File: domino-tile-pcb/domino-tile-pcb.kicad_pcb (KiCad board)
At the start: 2 copper layers, 39 x 35 mm, 1 part

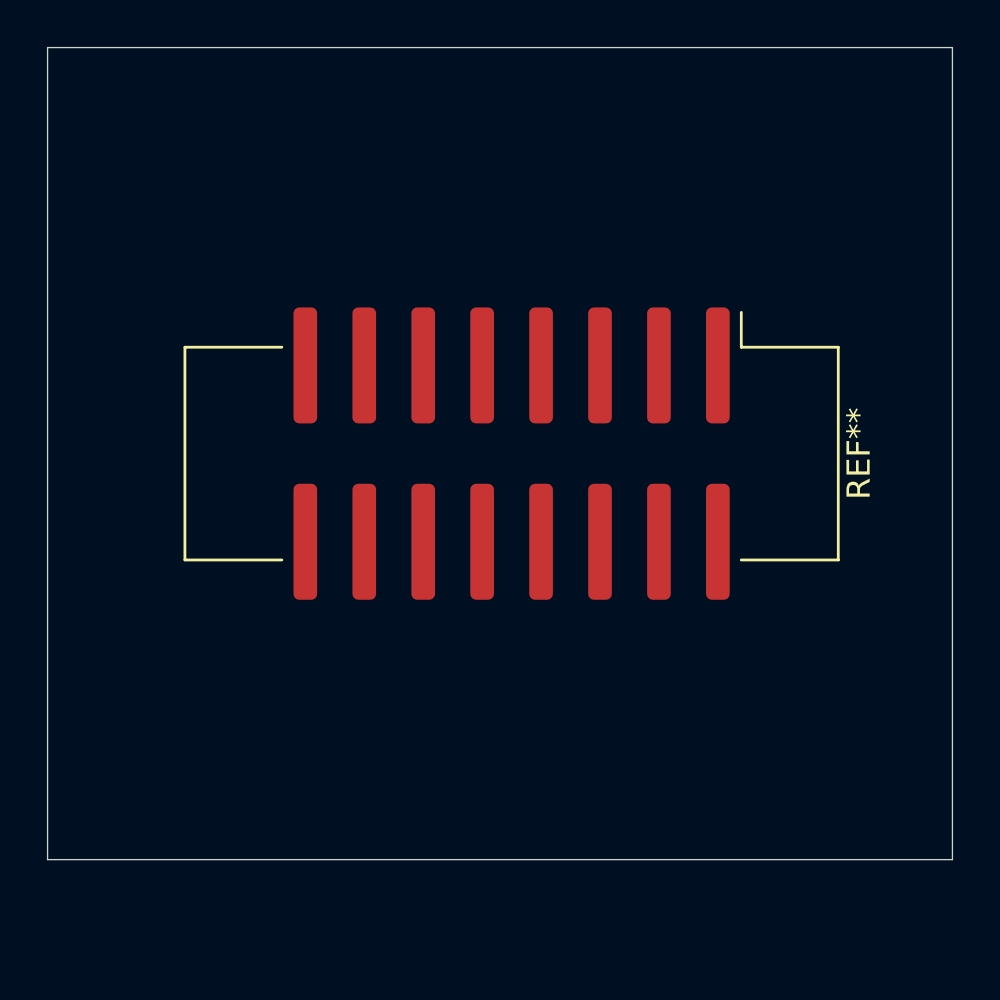
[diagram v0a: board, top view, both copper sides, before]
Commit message: do a lot of things, I guess
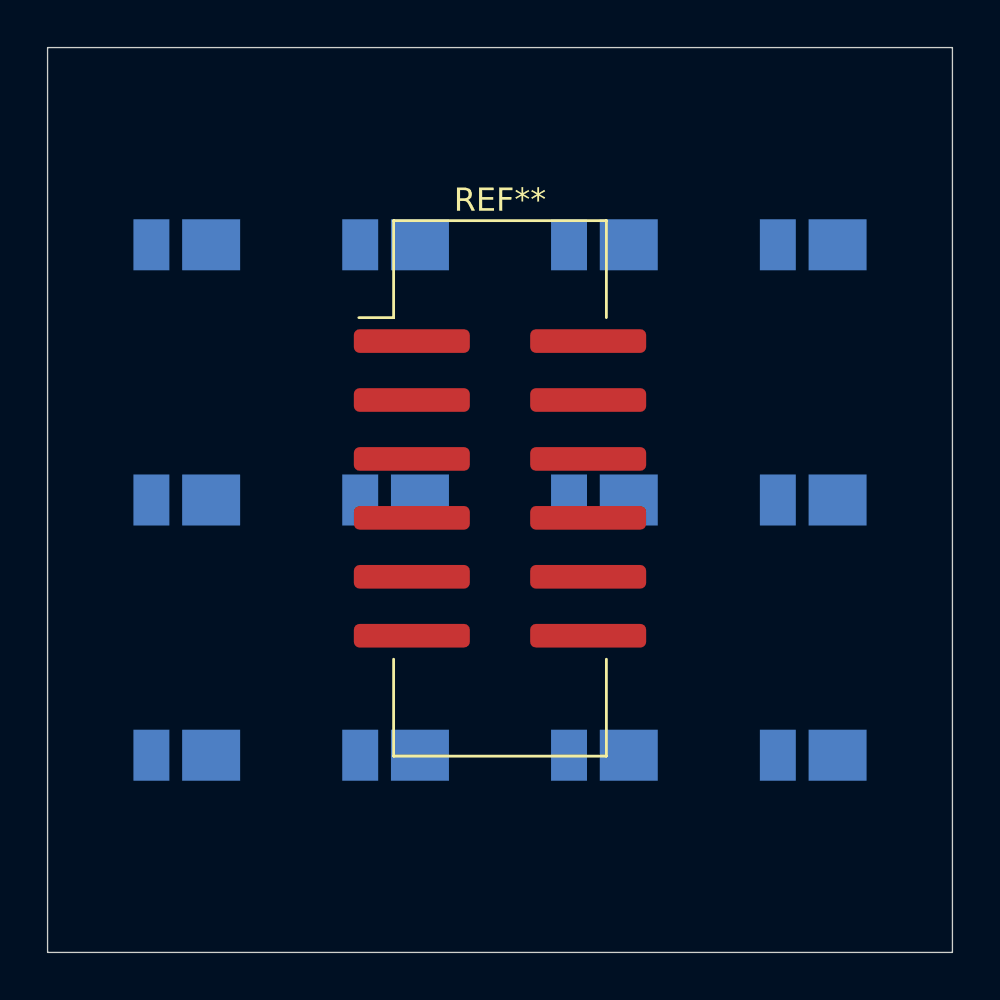
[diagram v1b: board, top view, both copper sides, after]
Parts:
- removed the REF** at (70.0, 67.5)
- added ?: 1, LED_SMD:LED_PLCC_2835_Handsoldering, B.Cu at (56.0, 69.5)
- added ?: 1, LED_SMD:LED_PLCC_2835_Handsoldering, B.Cu at (83.0, 58.5)
- added ?: 1, LED_SMD:LED_PLCC_2835_Handsoldering, B.Cu at (56.0, 58.5)
- added ?: 1, LED_SMD:LED_PLCC_2835_Handsoldering, B.Cu at (74.0, 58.5)
- added ?: 1, LED_SMD:LED_PLCC_2835_Handsoldering, B.Cu at (56.0, 80.5)
- added ?: 1, LED_SMD:LED_PLCC_2835_Handsoldering, B.Cu at (65.0, 58.5)
- added ?: 1, LED_SMD:LED_PLCC_2835_Handsoldering, B.Cu at (74.0, 80.5)
- added ?: 1, LED_SMD:LED_PLCC_2835_Handsoldering, B.Cu at (65.0, 69.5)
- added ?: 1, LED_SMD:LED_PLCC_2835_Handsoldering, B.Cu at (65.0, 80.5)
- added ?: 1, LED_SMD:LED_PLCC_2835_Handsoldering, B.Cu at (83.0, 80.5)
- added ?: 1, LED_SMD:LED_PLCC_2835_Handsoldering, B.Cu at (74.0, 69.5)
- added ?: 1, LED_SMD:LED_PLCC_2835_Handsoldering, B.Cu at (83.0, 69.5)
- added REF**: IDC-Header_2x06_P2.54mm_Vertical_SMD, Connector_IDC:IDC-Header_2x06_P2.54mm_Vertical_SMD, F.Cu at (69.5, 69.0)
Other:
- board size 39 x 35 mm -> 39 x 39 mm

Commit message: do more things
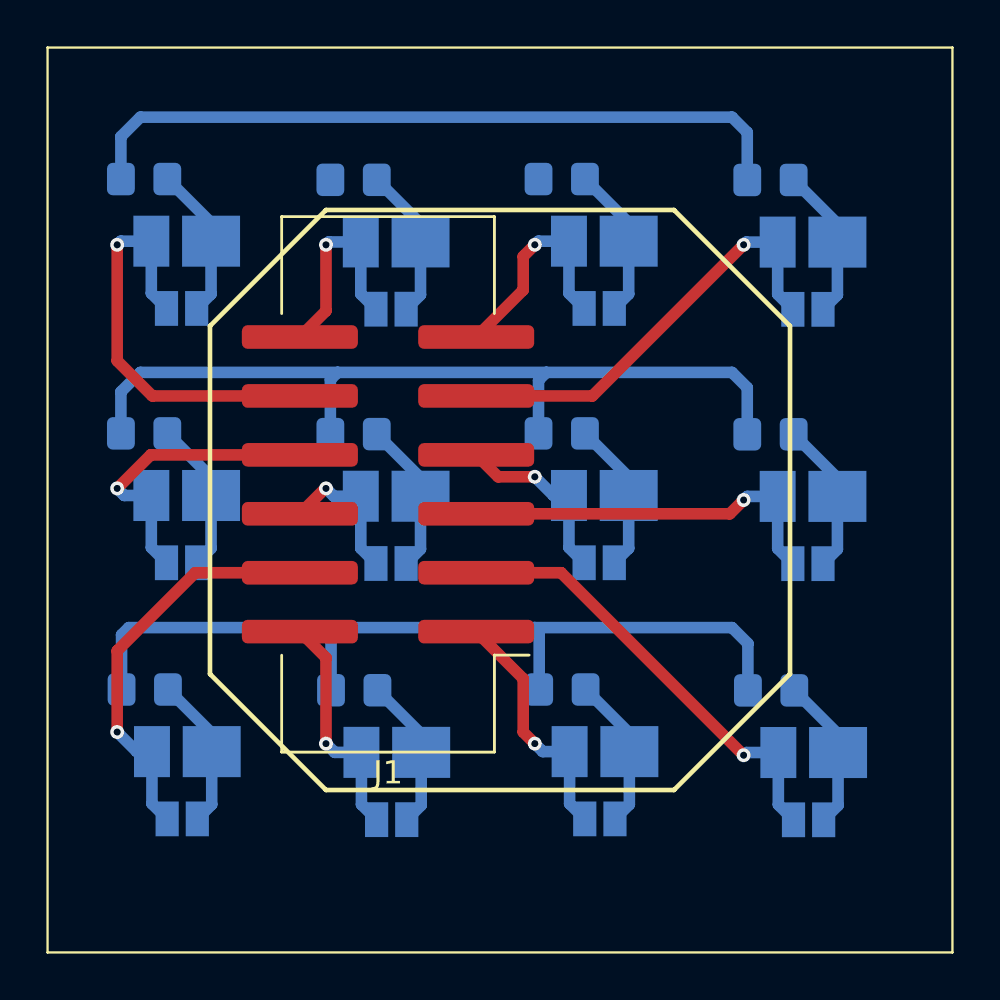
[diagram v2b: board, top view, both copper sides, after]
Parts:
- removed ? (x12): 1, LED_SMD:LED_PLCC_2835_Handsoldering
- added D1: ~, LED_SMD:LED_PLCC_2835_Handsoldering, B.Cu at (56.0, 80.3)
- added D10: ~, LED_SMD:LED_PLCC_2835_Handsoldering, B.Cu at (65.0, 58.4)
- added D11: ~, LED_SMD:LED_PLCC_2835_Handsoldering, B.Cu at (74.0, 58.3)
- added D12: ~, LED_SMD:LED_PLCC_2835_Handsoldering, B.Cu at (83.0, 58.4)
- added D2: ~, LED_SMD:LED_PLCC_2835_Handsoldering, B.Cu at (65.1, 80.4)
- added D3: ~, LED_SMD:LED_PLCC_2835_Handsoldering, B.Cu at (74.0, 80.3)
- added D4: ~, LED_SMD:LED_PLCC_2835_Handsoldering, B.Cu at (83.0, 80.4)
- added D5: ~, LED_SMD:LED_PLCC_2835_Handsoldering, B.Cu at (56.0, 69.3)
- added D6: ~, LED_SMD:LED_PLCC_2835_Handsoldering, B.Cu at (65.0, 69.3)
- added D7: ~, LED_SMD:LED_PLCC_2835_Handsoldering, B.Cu at (74.0, 69.3)
- added D8: ~, LED_SMD:LED_PLCC_2835_Handsoldering, B.Cu at (83.0, 69.3)
- added D9: ~, LED_SMD:LED_PLCC_2835_Handsoldering, B.Cu at (56.0, 58.3)
- added JP1: ~, Jumper:SolderJumper-2_P1.3mm_Open_Pad1.0x1.5mm, B.Cu at (55.8, 83.2)
- added JP10: ~, Jumper:SolderJumper-2_P1.3mm_Open_Pad1.0x1.5mm, B.Cu at (64.8, 61.3)
- added JP11: ~, Jumper:SolderJumper-2_P1.3mm_Open_Pad1.0x1.5mm, B.Cu at (73.8, 61.2)
- added JP12: ~, Jumper:SolderJumper-2_P1.3mm_Open_Pad1.0x1.5mm, B.Cu at (82.8, 61.3)
- added JP2: ~, Jumper:SolderJumper-2_P1.3mm_Open_Pad1.0x1.5mm, B.Cu at (64.8, 83.3)
- added JP3: ~, Jumper:SolderJumper-2_P1.3mm_Open_Pad1.0x1.5mm, B.Cu at (73.8, 83.2)
- added JP4: ~, Jumper:SolderJumper-2_P1.3mm_Open_Pad1.0x1.5mm, B.Cu at (82.8, 83.3)
- added JP5: ~, Jumper:SolderJumper-2_P1.3mm_Open_Pad1.0x1.5mm, B.Cu at (55.8, 72.2)
- added JP6: ~, Jumper:SolderJumper-2_P1.3mm_Open_Pad1.0x1.5mm, B.Cu at (64.8, 72.2)
- added JP7: ~, Jumper:SolderJumper-2_P1.3mm_Open_Pad1.0x1.5mm, B.Cu at (73.8, 72.2)
- added JP8: ~, Jumper:SolderJumper-2_P1.3mm_Open_Pad1.0x1.5mm, B.Cu at (82.8, 72.2)
- added JP9: ~, Jumper:SolderJumper-2_P1.3mm_Open_Pad1.0x1.5mm, B.Cu at (55.8, 61.2)
- added R1: 470, Resistor_SMD:R_0805_2012Metric_Pad1.20x1.40mm_HandSolder, B.Cu at (54.2, 77.7)
- added R10: 470, Resistor_SMD:R_0805_2012Metric_Pad1.20x1.40mm_HandSolder, B.Cu at (63.2, 55.7)
- added R11: 470, Resistor_SMD:R_0805_2012Metric_Pad1.20x1.40mm_HandSolder, B.Cu at (72.2, 55.7)
- added R12: 470, Resistor_SMD:R_0805_2012Metric_Pad1.20x1.40mm_HandSolder, B.Cu at (81.2, 55.7)
- added R2: 470, Resistor_SMD:R_0805_2012Metric_Pad1.20x1.40mm_HandSolder, B.Cu at (63.2, 77.7)
- added R3: 470, Resistor_SMD:R_0805_2012Metric_Pad1.20x1.40mm_HandSolder, B.Cu at (72.2, 77.7)
- added R4: 470, Resistor_SMD:R_0805_2012Metric_Pad1.20x1.40mm_HandSolder, B.Cu at (81.2, 77.7)
- added R5: 470, Resistor_SMD:R_0805_2012Metric_Pad1.20x1.40mm_HandSolder, B.Cu at (54.2, 66.6)
- added R6: 470, Resistor_SMD:R_0805_2012Metric_Pad1.20x1.40mm_HandSolder, B.Cu at (63.2, 66.7)
- added R7: 470, Resistor_SMD:R_0805_2012Metric_Pad1.20x1.40mm_HandSolder, B.Cu at (72.2, 66.6)
- added R8: 470, Resistor_SMD:R_0805_2012Metric_Pad1.20x1.40mm_HandSolder, B.Cu at (81.2, 66.7)
- added R9: 470, Resistor_SMD:R_0805_2012Metric_Pad1.20x1.40mm_HandSolder, B.Cu at (54.2, 55.7)
- J1: renamed from REF**; value IDC-Header_2x06_P2.54mm_Vertical_SMD -> ~
- moved J1 4.83 mm to (64.7, 68.8), turned to 180 degrees
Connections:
- J1 pad 1: (no net) -> Net-(D3-A)
- J1 pad 10: (no net) -> Net-(D9-A)
- J1 pad 11: (no net) -> Net-(D11-A)
- J1 pad 12: (no net) -> Net-(D10-A)
- J1 pad 2: (no net) -> Net-(D2-A)
- J1 pad 3: (no net) -> Net-(D4-A)
- J1 pad 4: (no net) -> Net-(D1-A)
- J1 pad 5: (no net) -> Net-(D8-A)
- J1 pad 6: (no net) -> Net-(D6-A)
- J1 pad 7: (no net) -> Net-(D7-A)
- J1 pad 8: (no net) -> Net-(D5-A)
- J1 pad 9: (no net) -> Net-(D12-A)
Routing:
- net GND: track 0.00 -> 105.8 mm
- net Net-(D4-A): track 0.00 -> 19.5 mm, vias 0 -> 1
- net Net-(D12-A): track 0.00 -> 18.9 mm, vias 0 -> 1
- net Net-(D9-A): track 0.00 -> 18.2 mm, vias 0 -> 1
- net Net-(D1-A): track 0.00 -> 17.8 mm, vias 0 -> 1
- net Net-(D8-A): track 0.00 -> 16.5 mm, vias 0 -> 1
- net Net-(D5-A): track 0.00 -> 13.2 mm, vias 0 -> 1
- net Net-(D3-A): track 0.00 -> 10.7 mm, vias 0 -> 1
- net Net-(D2-A): track 0.00 -> 10.1 mm, vias 0 -> 1
- net Net-(D11-A): track 0.00 -> 9.73 mm, vias 0 -> 1
- net Net-(D10-A): track 0.00 -> 9.16 mm, vias 0 -> 1
- net Net-(D7-A): track 0.00 -> 7.89 mm, vias 0 -> 1
- net Net-(D12-K): track 0.00 -> 7.01 mm
- net Net-(D6-K): track 0.00 -> 7.01 mm
- net Net-(D1-K): track 0.00 -> 7.01 mm
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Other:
- board outline removed
